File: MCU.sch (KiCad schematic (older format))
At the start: 30 parts

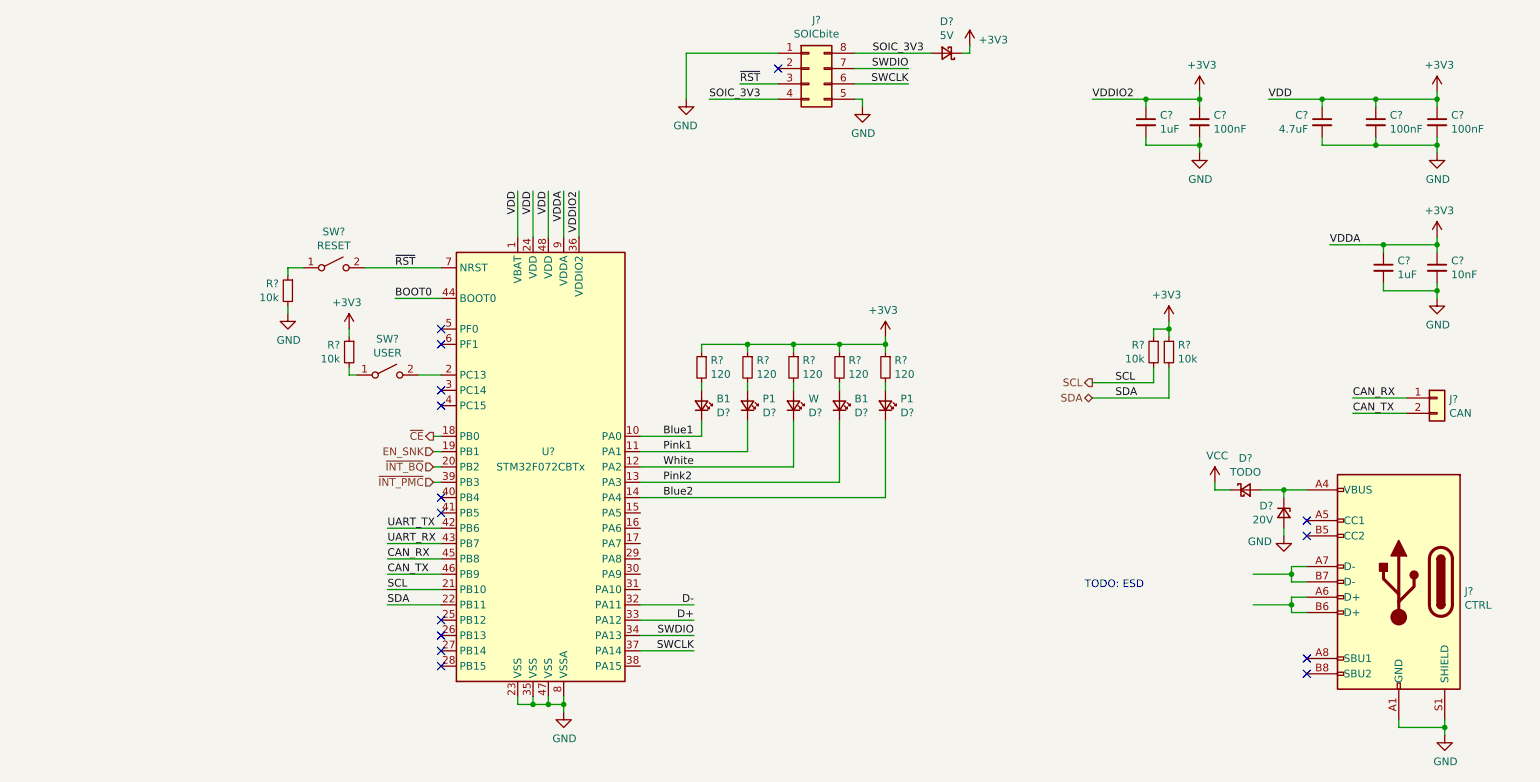
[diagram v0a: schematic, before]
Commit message: almost done
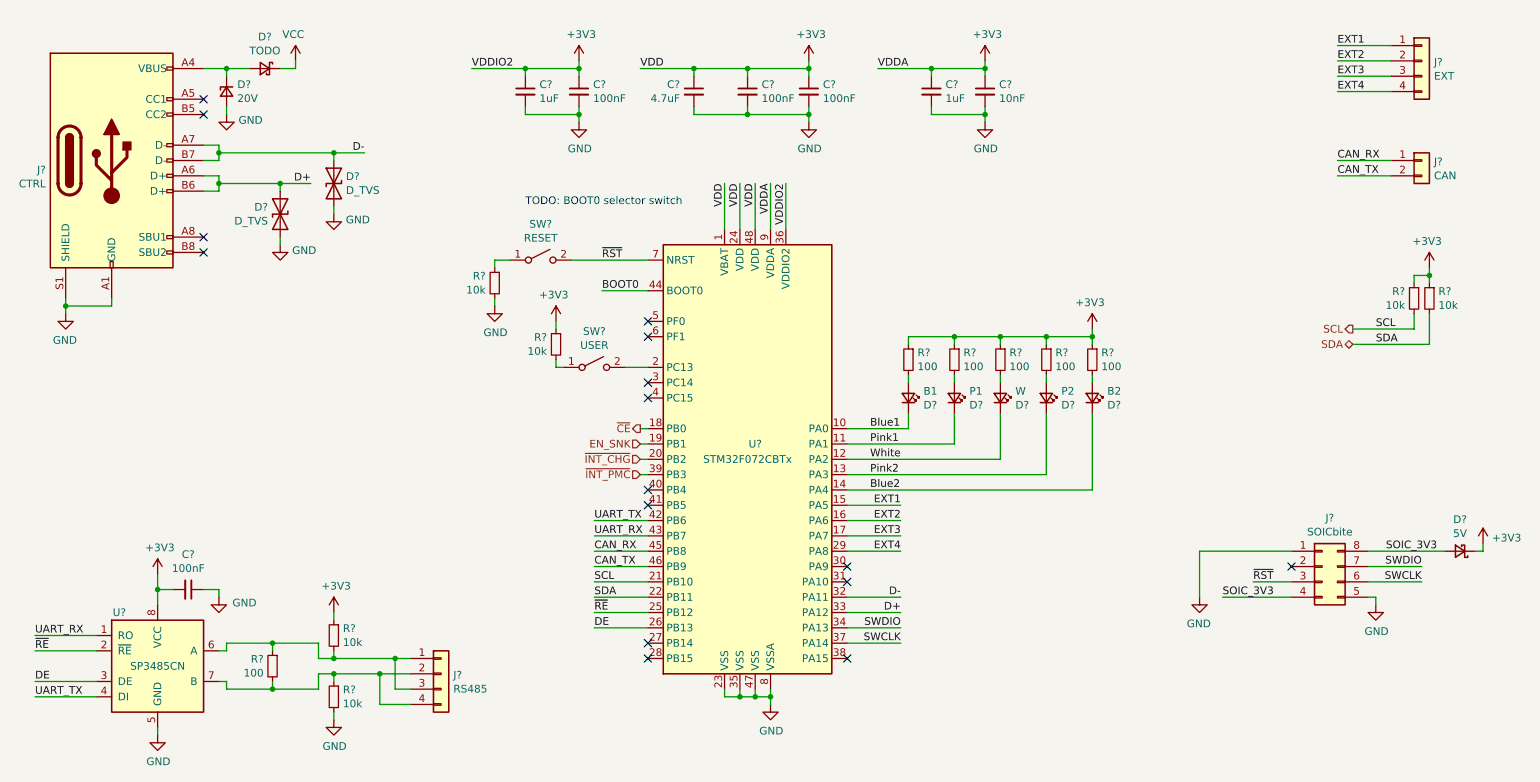
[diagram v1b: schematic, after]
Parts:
- removed D?: B1, symbol Device:LED_Small
- removed D?: P1, symbol Device:LED_Small
- added C?: 100nF, Capacitor_SMD:C_0603_1608Metric, symbol Device:C_Small
- added D? (x2): D_TVS, symbol Device:D_TVS
- added D?: P2, LED_SMD:LED_0603_1608Metric_Castellated, symbol Device:LED_Small
- added D?: B2, LED_SMD:LED_0603_1608Metric_Castellated, symbol Device:LED_Small
- added J?: RS485, symbol Connector_Generic:Conn_01x04
- added J?: EXT, symbol Connector_Generic:Conn_01x04
- added R? (x2): 10k, Resistor_SMD:R_0603_1608Metric, symbol Device:R_Small
- added R?: 100, Resistor_SMD:R_0603_1608Metric, symbol Device:R_Small
- added U?: SP3485CN, Package_SO:SOIC-8_3.9x4.9mm_P1.27mm, symbol Interface_UART:SP3485CN
- D?: footprint (none) -> LED_SMD:LED_0603_1608Metric_Castellated; MPN (none) -> OSB60603C1E
- D?: footprint (none) -> LED_SMD:LED_0603_1608Metric_Castellated; MPN (none) -> OSK40603C1E
- D?: footprint (none) -> LED_SMD:LED_0603_1608Metric_Castellated; MPN (none) -> OSW50603C1E
- J?: footprint (none) -> Connector_USB:USB_C_Receptacle_HRO_TYPE-C-31-M-12
- R? (x5): value 120 -> 100
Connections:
- net +3V3: now also C?.2, R?.1, U?.8 (VCC)
- net Blue2: now also D?.1 (K)
- net D+: now also J?.A6 (D+), J?.B6 (D+), D?.1 (A1)
- net D-: now also J?.A7 (D-), J?.B7 (D-), D?.1 (A1)
- net GND: now also C?.1, D?.2 (A2), D?.2 (A2), R?.2, U?.5 (GND)
- net Pink2: now also D?.1 (K)
- net UART_RX: now also U?.1 (RO)
- net UART_TX: now also U?.4 (DI)
- net EXT1: now reaches U?.15 (PA5)
- net EXT1: now also J?.1 (Pin_1)
- net EXT2: now reaches U?.16 (PA6)
- net EXT2: now also J?.2 (Pin_2)
- net EXT3: now reaches U?.17 (PA7)
- net EXT3: now also J?.3 (Pin_3)
- net ~RE: now reaches U?.25 (PB12)
- net ~RE: now also U?.2 (~RE~)
- net DE: now reaches U?.26 (PB13)
- net DE: now also U?.3 (DE)
- net EXT4: now reaches U?.29 (PA8)
- net EXT4: now also J?.4 (Pin_4)
- net at R?.2: now also D?.2 (A) (x2)
- net ~INT_BQ renamed ~INT_CHG
- new net: J?.1 (Pin_1), J?.3 (Pin_3), R?.1, R?.2, U?.6 (A)
- new net: J?.2 (Pin_2), J?.4 (Pin_4), R?.1, R?.2, U?.7 (B)
- no-connect marks 15 -> 16
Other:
- note added: "TODO: BOOT0 selector switch"
- note removed: "TODO: ESD"
- moved on the sheet: C?, D?, J?, R?, SW?, U?
